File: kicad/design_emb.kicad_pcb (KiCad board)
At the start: 2 copper layers, 107 parts, among them J1 Conn_01x03, J2 Barrel_Jack, J3 USB_A, J4 Conn_01x03, J5 Conn_02x11_Counter_Clockwise, J6 Conn_02x10_Counter_Clockwise, J7 Screw_Terminal_01x02, J8 Screw_Terminal_01x02, K1 SANYOU_SRD_Form_C, K2 SANYOU_SRD_Form_C, Q1 MMBT3904, Q2 MMBT3904, U1 SRX.X.TCT, U10 S25FL116KOXNFIQ-11, U2 SRX.X.TCT, U3 STM32F446ZETx, U4 ICE40HX1K, U5 TLV1117LV33DCYR, U6 TLV1117LV33DCYR, U7 TLV1117LV12DCYR, U8 OMEGA2, U9 RCLAMP0502B

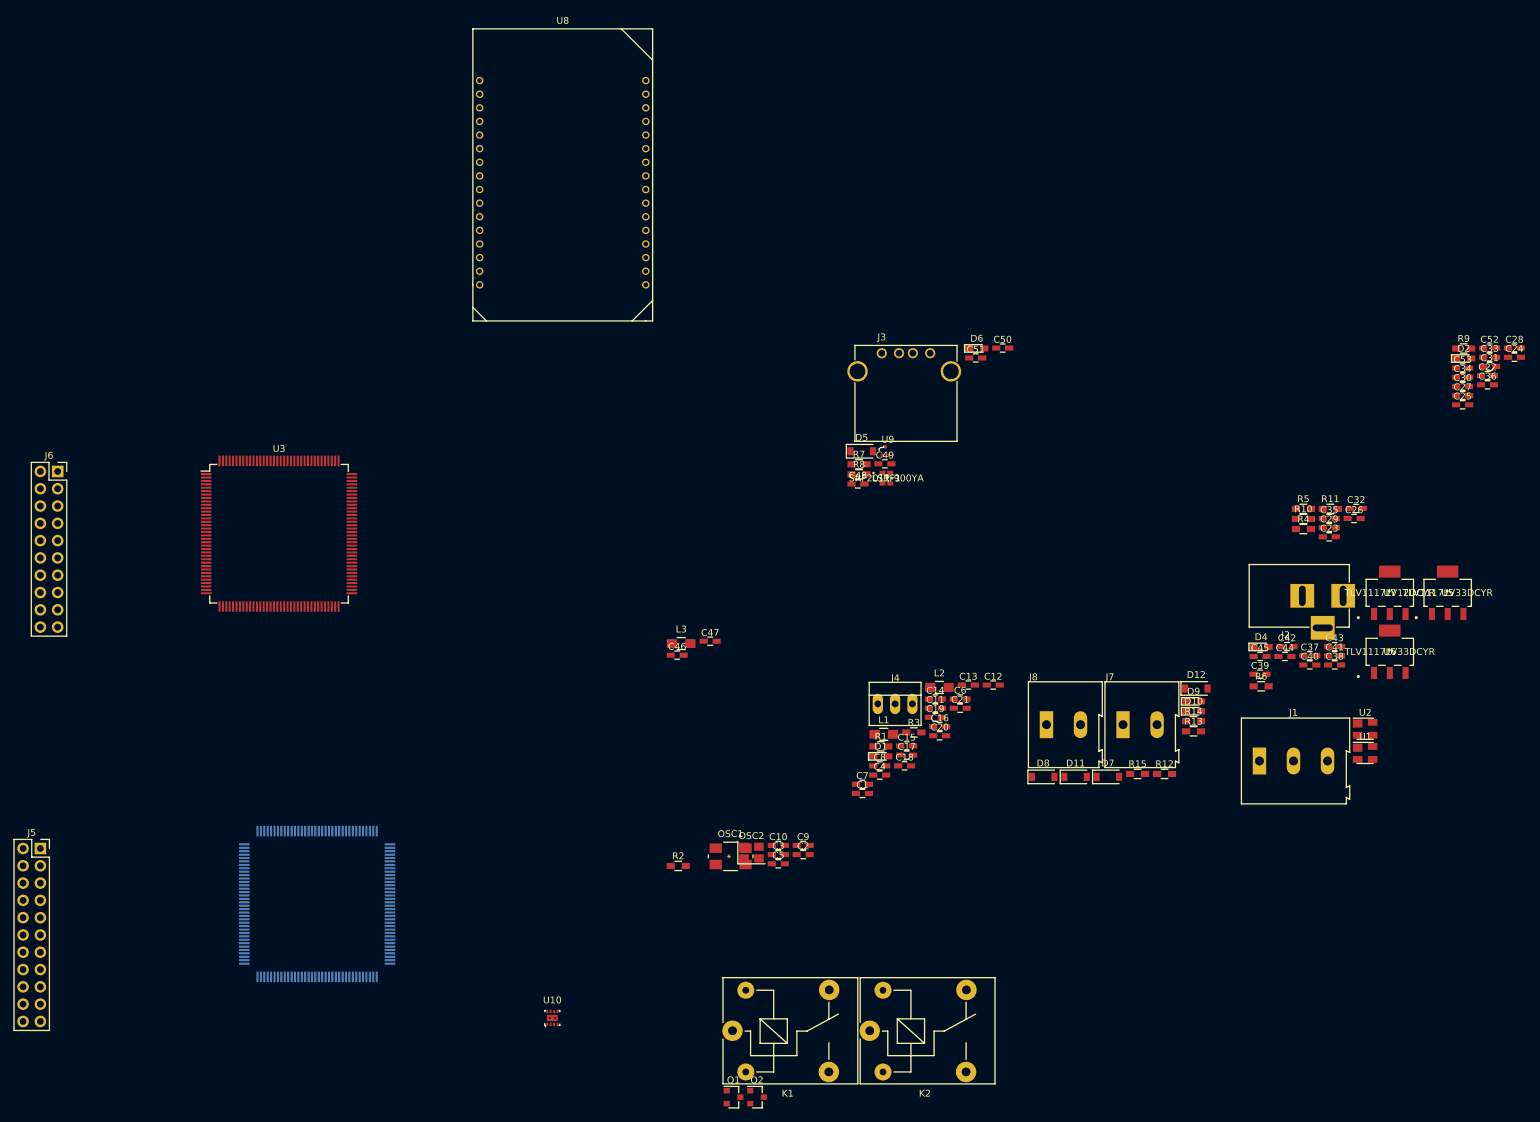
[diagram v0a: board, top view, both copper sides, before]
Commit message: design_emb.ses
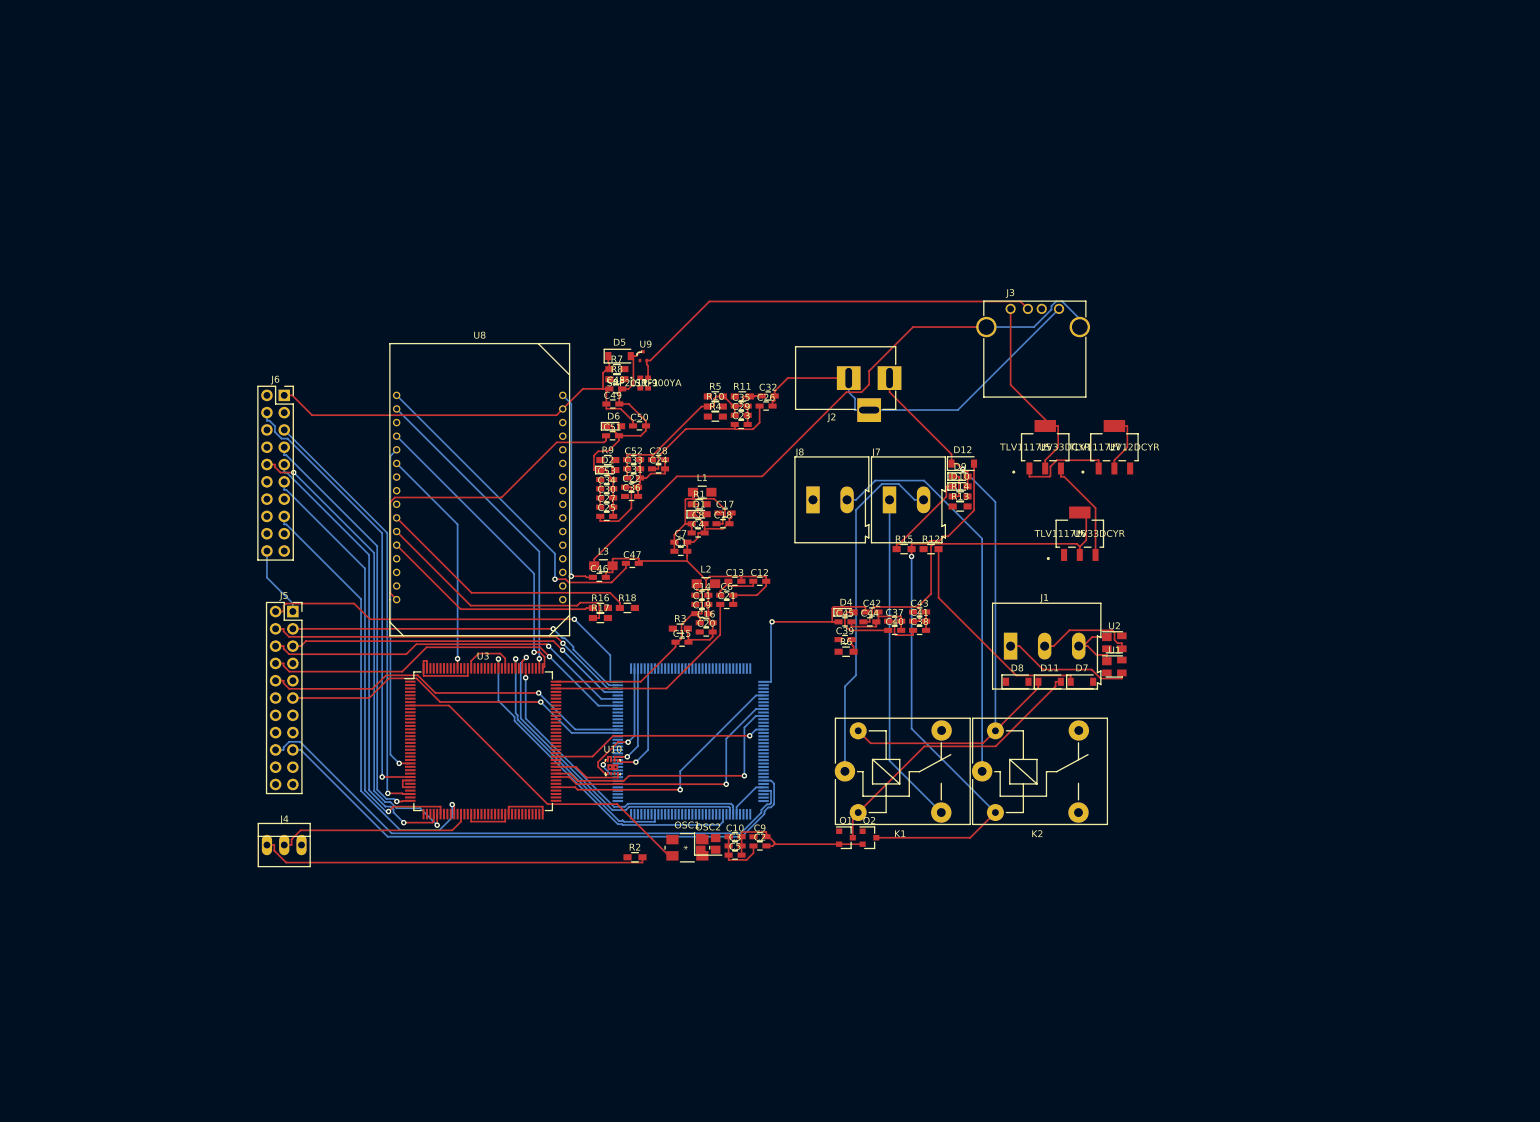
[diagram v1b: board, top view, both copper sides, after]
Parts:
- added R16: 100, Resistors_SMD:R_0603_HandSoldering, F.Cu at (108.7, 117.6)
- added R17: 100, Resistors_SMD:R_0603_HandSoldering, F.Cu at (108.7, 119.1)
- added R18: 100, Resistors_SMD:R_0603_HandSoldering, F.Cu at (112.6, 117.6)
- R11: value 10k -> 4.7k
- R9: value 10k -> 100
- moved C25 126.8 mm to (109.6, 104.1)
- moved C27 126.8 mm to (109.6, 102.8)
- moved C30 126.8 mm to (109.6, 101.4)
- moved C34 126.8 mm to (109.6, 100.1)
- moved C53 126.8 mm to (109.6, 98.7)
- moved D2 126.8 mm to (109.8, 97.3)
- moved R9 126.8 mm to (109.8, 95.9)
- moved C22 126.8 mm to (113.2, 99.8)
- moved C24 126.8 mm to (117.2, 97.2)
- moved C28 126.8 mm to (117.2, 95.8)
- moved C31 126.8 mm to (113.5, 98.5)
- moved C33 126.8 mm to (113.5, 97.2)
- moved C36 126.8 mm to (113.2, 101.2)
- moved C52 126.8 mm to (113.5, 95.8)
- moved J4 92.1 mm to (59.7, 152.4)
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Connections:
- R10 pad 2: /Sheet2/SPI3 -> /sheet3/SPI0
- R11 pad 1: /Sheet2/SPI1 -> /sheet3/SPI1
- R12 pad 1: Net-(Q1-Pad1) -> Net-(R12-Pad1)
- R13 pad 1: Net-(Q2-Pad1) -> Net-(R13-Pad1)
- R9 pad 1: /Sheet2/SPI2 -> Net-(R9-Pad1)
- R9 pad 2: /Sheet4/+3V3_FPGA -> /Sheet2/SPI0
- U10 pad 1: /Sheet2/SPI0 -> /sheet3/SPI0
- U10 pad 2: /Sheet2/SPI2 -> /sheet3/SPI2
- U10 pad 5: /Sheet2/SPI3 -> /sheet3/SPI3
- U10 pad 6: /Sheet2/SPI1 -> /sheet3/SPI1
- U4 pad 112: /Sheet1/FMCNBL0 -> /sheet3/FMCNBL0
- U4 pad 113: /Sheet1/FMCNBL1 -> /sheet3/FMCNBL1
- U4 pad 67: /Sheet2/SPI3 -> /sheet3/SPI3
- U4 pad 68: /Sheet2/SPI2 -> /sheet3/SPI2
- U4 pad 70: /Sheet2/SPI1 -> /sheet3/SPI1
- U4 pad 71: /Sheet2/SPI0 -> /sheet3/SPI0
- U8 pad 10: /Sheet2/SPI3 -> Net-(R18-Pad1)
- U8 pad 11: /Sheet2/SPI2 -> Net-(R17-Pad1)
- U8 pad 12: /Sheet2/SPI1 -> Net-(R16-Pad1)
- U8 pad 13: /Sheet2/SPI0 -> Net-(R9-Pad1)
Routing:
- net GND: track 0.00 -> 285.0 mm
- net VDD: track 0.00 -> 195.6 mm
- net /Sheet4/+3V3_FPGA: track 0.00 -> 93.4 mm, vias 0 -> 1
- net +5VA: track 0.00 -> 93.3 mm, vias 0 -> 1
- net Net-(J3-Pad5): track 0.00 -> 91.7 mm
- net /sheet3/GPIO3: track 0.00 -> 84.0 mm
- net /sheet3/GPIO4: track 0.00 -> 82.9 mm
- net Net-(D12-Pad2): track 0.00 -> 81.8 mm, vias 0 -> 1
- net /Sheet1/USR9: track 0.00 -> 69.3 mm, vias 0 -> 2
- net /Sheet4/+1V2_FPGA: track 0.00 -> 69.2 mm, vias 0 -> 1
- net /Sheet1/USR8: track 0.00 -> 66.1 mm, vias 0 -> 1
- net /Sheet1/USR3: track 0.00 -> 65.4 mm, vias 0 -> 1
- net /Sheet1/USR14: track 0.00 -> 65.1 mm, vias 0 -> 1
- net /Sheet1/USR10: track 0.00 -> 64.2 mm, vias 0 -> 1
- net /Sheet1/USR4: track 0.00 -> 63.0 mm, vias 0 -> 1
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
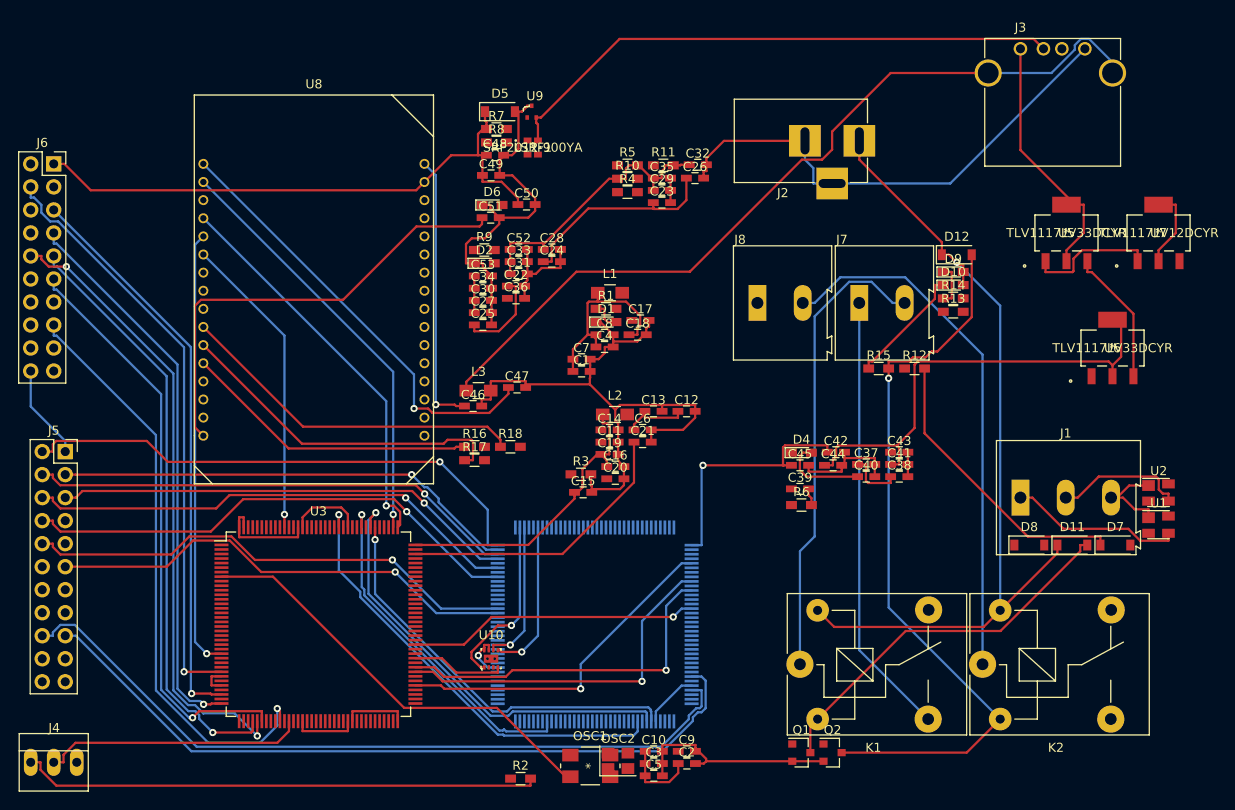
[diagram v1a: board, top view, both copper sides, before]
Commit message: design_emb.kicad_pcb
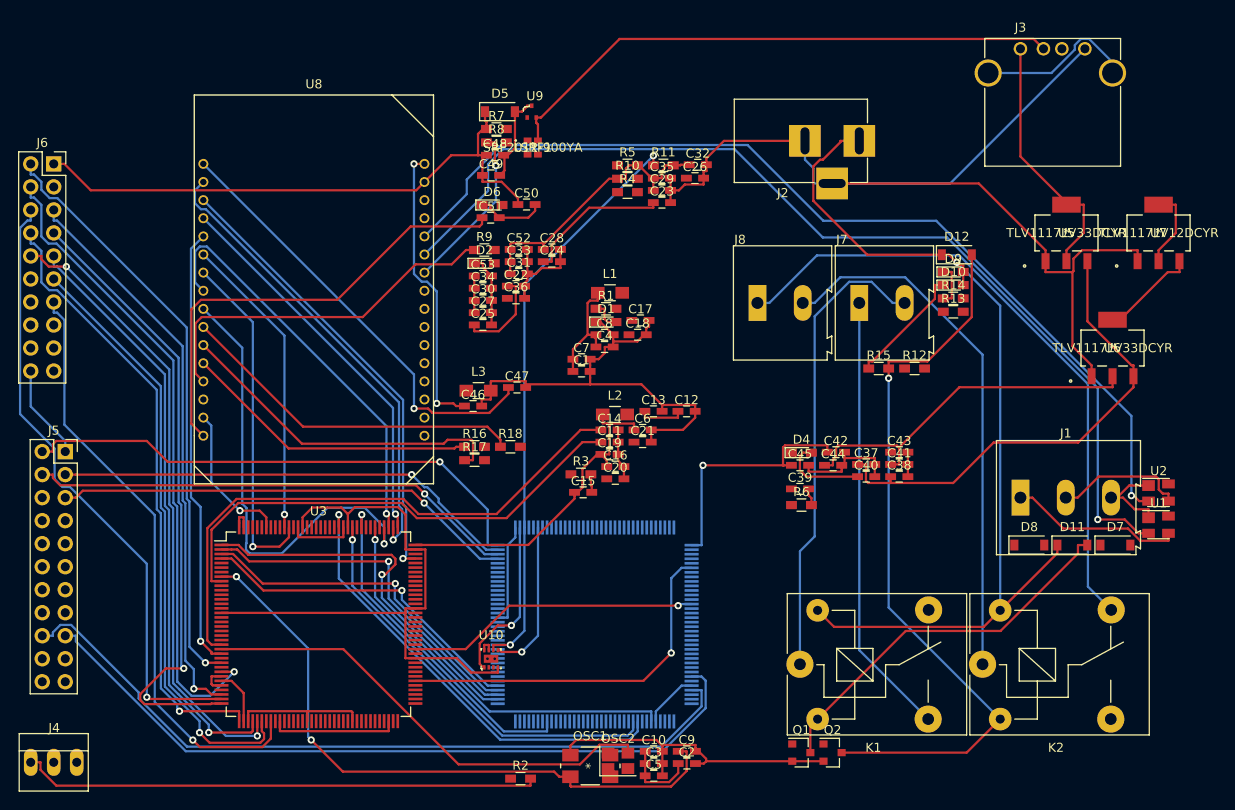
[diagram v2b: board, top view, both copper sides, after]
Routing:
- net /SERIAL_RX: track 0.00 -> 112.5 mm, vias 0 -> 1
- net /SERIAL_TX: track 0.00 -> 106.4 mm, vias 0 -> 1
- net GND: track 285.0 -> 367.4 mm
- net Net-(J3-Pad5): track 91.7 -> 17.8 mm
- net Net-(J8-Pad1): track 0.00 -> 70.5 mm
- net /Sheet1/USR5: track 0.00 -> 69.1 mm, vias 0 -> 1
- net /Sheet1/USR7: track 0.00 -> 68.0 mm, vias 0 -> 1
- net /Sheet1/USR12: track 0.00 -> 66.2 mm, vias 0 -> 1
- net /Sheet1/USR1: track 0.00 -> 65.5 mm, vias 0 -> 1
- net /Sheet1/OSC_IN: track 0.00 -> 63.5 mm
- net /sheet3/GPIO16: track 56.0 -> 0.00 mm, vias 1 -> 0
- net /Sheet1/OSC32_OUT: track 0.00 -> 55.1 mm
- net /sheet3/GPIO18: track 55.1 -> 0.00 mm, vias 1 -> 0
- net /sheet3/GPIO14: track 54.9 -> 0.00 mm, vias 1 -> 0
- net /sheet3/GPIO19: track 52.2 -> 0.00 mm, vias 1 -> 0
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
